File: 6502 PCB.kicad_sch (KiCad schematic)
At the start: 9 parts, among them SW1 RESET, U1 W65C02SxP, U2 28C256, U3 CY62256-70PC, U4 W65C22NxP, X1 1MHz

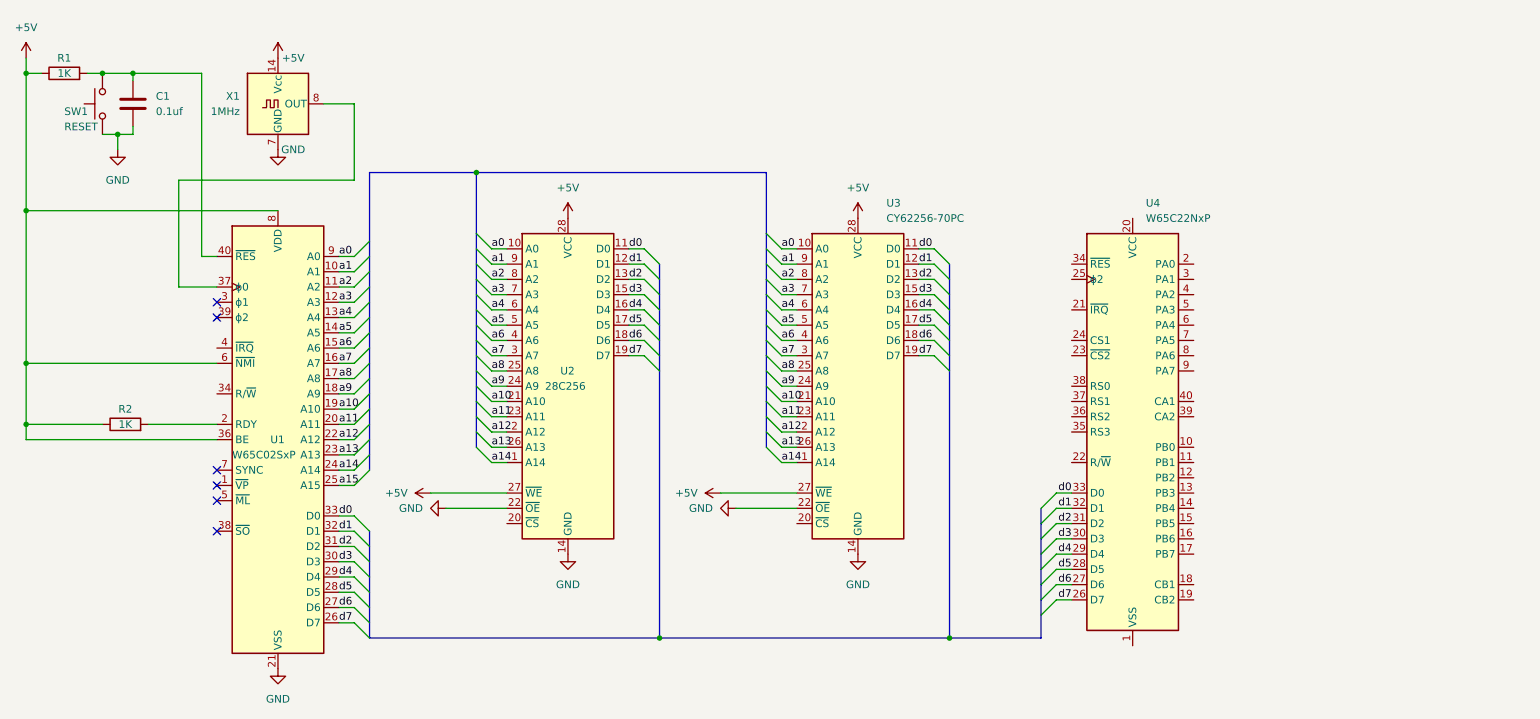
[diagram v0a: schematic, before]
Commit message: think i finished schematic
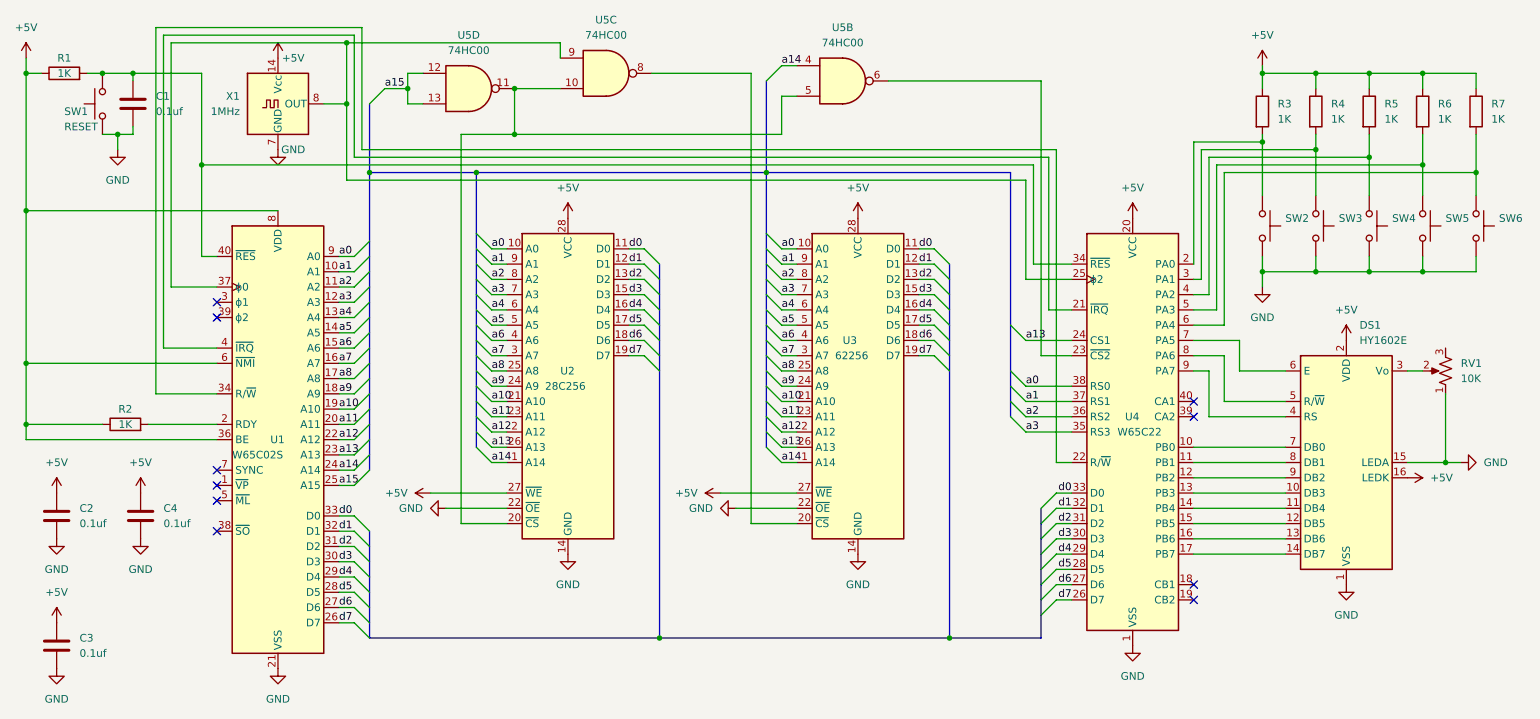
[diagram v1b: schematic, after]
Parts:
- added C2, C3, C4: 0.1uf, Capacitor_SMD:CP_Elec_3x5.3, symbol Device:C
- added DS1: HY1602E, Display:HY1602E, symbol Display_Character:HY1602E
- added R3, R4, R5, R6, R7: 1K, Resistor_SMD:R_0201_0603Metric, symbol Device:R
- added RV1: 10K, Potentiometer_SMD:Potentiometer_ACP_CA6-VSMD_Vertical, symbol Device:R_Potentiometer_US
- added SW2, SW3, SW4, SW5, SW6: SW_Push, Button_Switch_SMD:SW_SPST_PTS645, symbol Switch:SW_Push
- added U5: 74HC00, Package_DIP:DIP-14_W7.62mm, symbol 74xx:74HC00
- C1: footprint (none) -> Capacitor_SMD:CP_Elec_3x5.3
- R1, R2: footprint (none) -> Resistor_SMD:R_0201_0603Metric
- SW1: footprint (none) -> Button_Switch_SMD:SW_SPST_PTS645
- U1: value W65C02SxP -> W65C02S
- U2: footprint (none) -> Package_DIP:DIP-28_W15.24mm
- U3: value CY62256-70PC -> 62256
- U4: value W65C22NxP -> W65C22
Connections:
- net +5V: now also U4.20 (VCC), C2.1, C3.1, C4.1, DS1.16 (LEDK), DS1.2 (VDD), R3.1, R4.1, R5.1, R6.1, R7.1
- net GND: now also U4.1 (VSS), C2.2, C3.2, C4.2, DS1.1 (VSS), DS1.15 (LEDA), RV1.1, SW2.2, SW3.2, SW4.2, SW5.2, SW6.2
- net a0: now also U4.38 (RS0)
- net a1: now also U4.37 (RS1)
- net a13: now also U4.24 (CS1)
- net a14: now also U5.4
- net a15: now also U5.12, U5.13
- net a2: now also U4.36 (RS2)
- net a3: now also U4.35 (RS3)
- net at C1.1, R1.2, SW1.2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: now also U4.34 (~{RES})
- net at U1.37 (ϕ0), X1.8 (OUT): now also U4.25 (ϕ2), U5.9
- net at U4.10 (PB0): now also DS1.7 (DB0)
- net at U4.11 (PB1): now also DS1.8 (DB1)
- net at U4.12 (PB2): now also DS1.9 (DB2)
- net at U4.13 (PB3): now also DS1.10 (DB3)
- net at U4.14 (PB4): now also DS1.11 (DB4)
- net at U4.15 (PB5): now also DS1.12 (DB5)
- net at U4.16 (PB6): now also DS1.13 (DB6)
- net at U4.17 (PB7): now also DS1.14 (DB7)
- net at U4.2 (PA0): now also R3.2, SW2.1
- net at U4.21 (~{IRQ}): now also U1.4 (~{IRQ})
- net at U4.22 (R/~{W}): now also U1.34 (R/~{W})
- net at U4.23 (~{CS2}): now also U5.6
- net at U4.3 (PA1): now also R4.2, SW3.1
- net at U4.4 (PA2): now also R5.2, SW4.1
- net at U4.5 (PA3): now also R6.2, SW5.1
- net at U4.6 (PA4): now also R7.2, SW6.1
- net at U4.7 (PA5): now also DS1.6 (E)
- net at U4.8 (PA6): now also DS1.5 (R/~{W})
- net at U4.9 (PA7): now also DS1.4 (RS)
- net at U3.20 (~{CS}): now also U5.8
- net at U2.20 (~{CS}): now also U5.10, U5.11, U5.5
- new net: DS1.3 (Vo), RV1.2
- no-connect marks 6 -> 10
